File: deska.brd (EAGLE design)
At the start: 98.7 x 80 mm, 5 parts

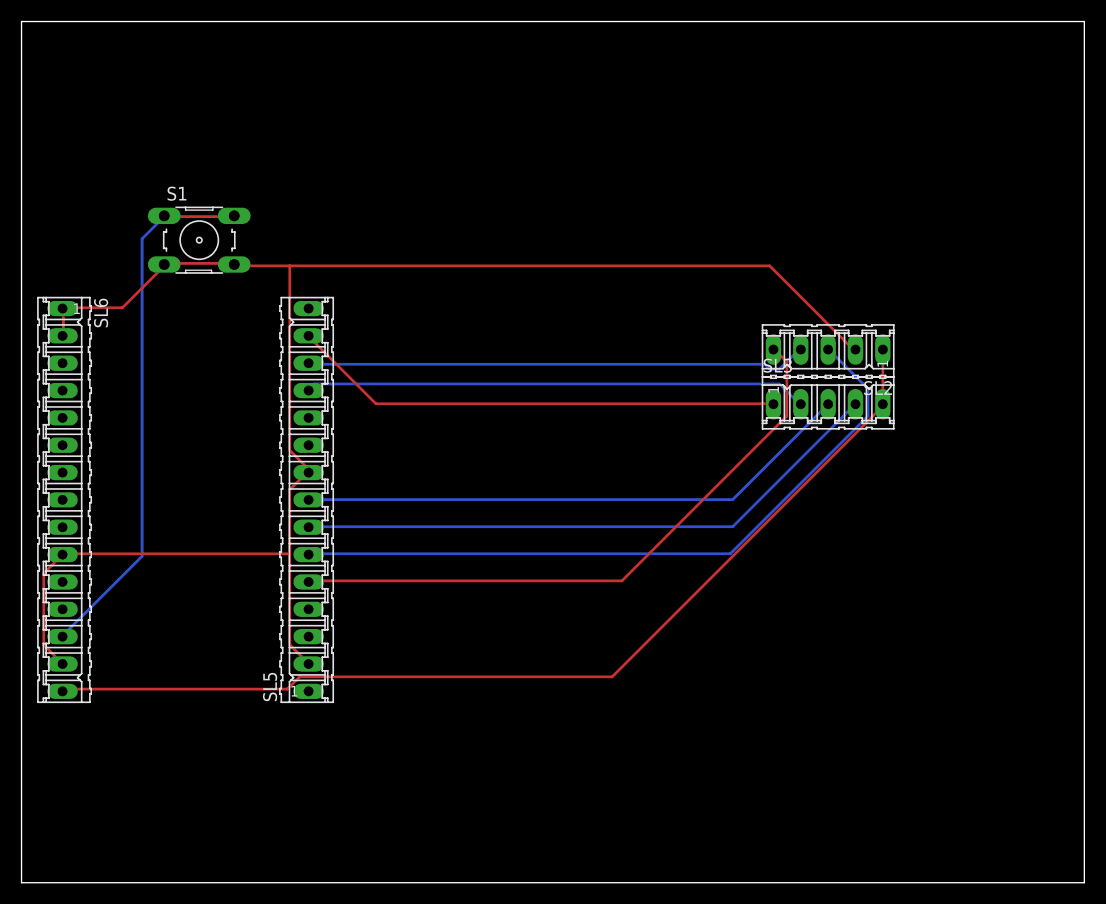
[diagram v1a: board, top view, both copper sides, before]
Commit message: uprava navrhu
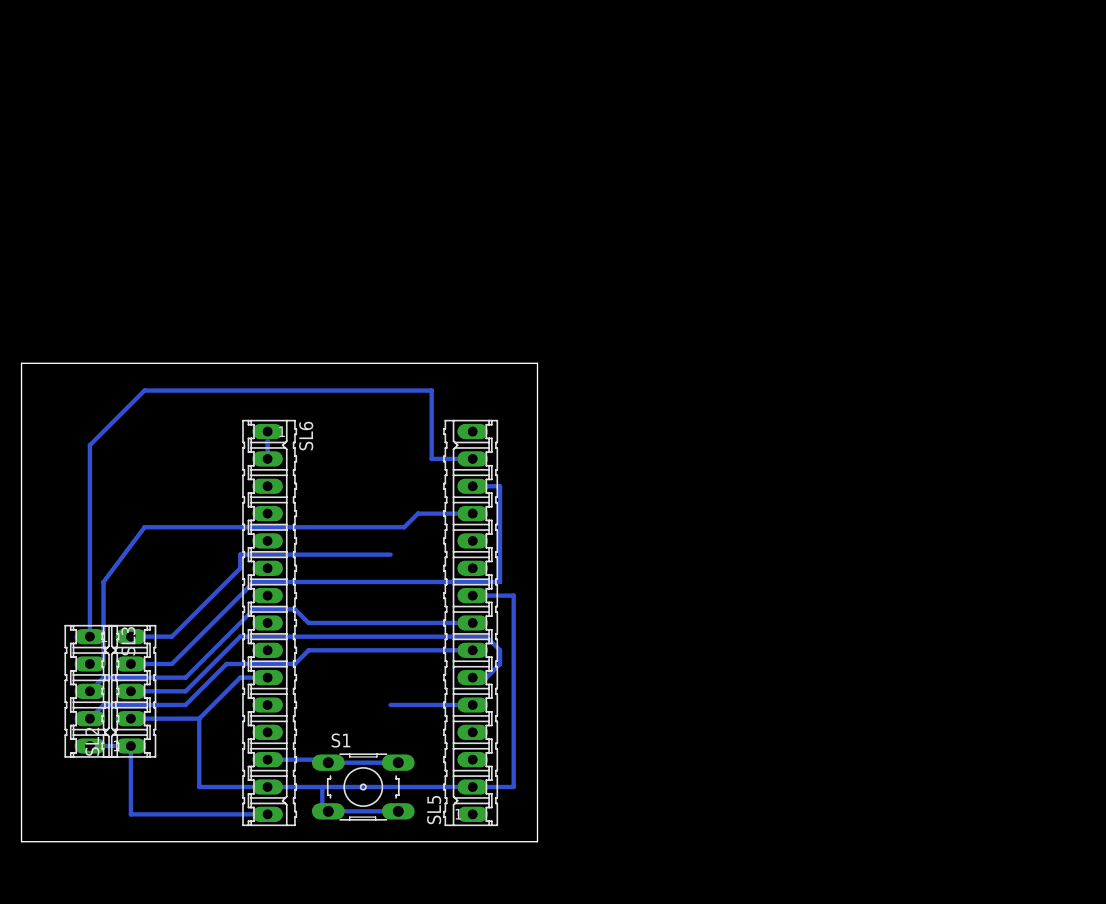
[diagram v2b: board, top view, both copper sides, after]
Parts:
- moved SL3 73.6 mm to (6.35, 14.0), turned to 270 degrees
- moved SL2 72.1 mm to (10.2, 14.0), turned to 90 degrees
- moved S1 53.0 mm to (31.8, 5.08)
- moved SL6 22.2 mm to (22.9, 20.3)
- moved SL5 19.0 mm to (41.9, 20.3)
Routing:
- net GND: track 153.4 -> 83.0 mm
- net +5V: track 92.5 -> 22.9 mm
- net N$10: track 49.6 -> 12.3 mm
- net N$6: track 65.0 -> 41.3 mm
- net N$2: track 57.6 -> 35.7 mm
- net N$7: track 55.5 -> 38.2 mm
- net N$1: track 45.8 -> 61.8 mm
- net N$5: track 51.9 -> 39.2 mm
- net N$4: track 46.7 -> 48.9 mm
- net N$3: track 46.8 -> 46.2 mm
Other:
- board size 98.7 x 80 mm -> 47.9 x 44.4 mm
